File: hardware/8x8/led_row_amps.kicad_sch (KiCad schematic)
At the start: 10 parts

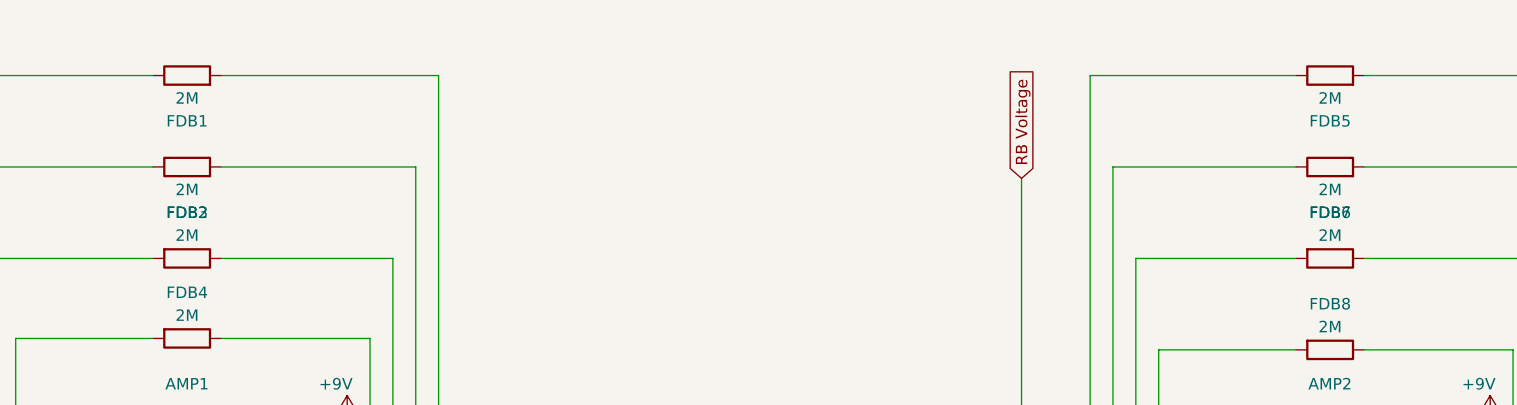
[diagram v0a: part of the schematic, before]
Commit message: Completed Major Routing
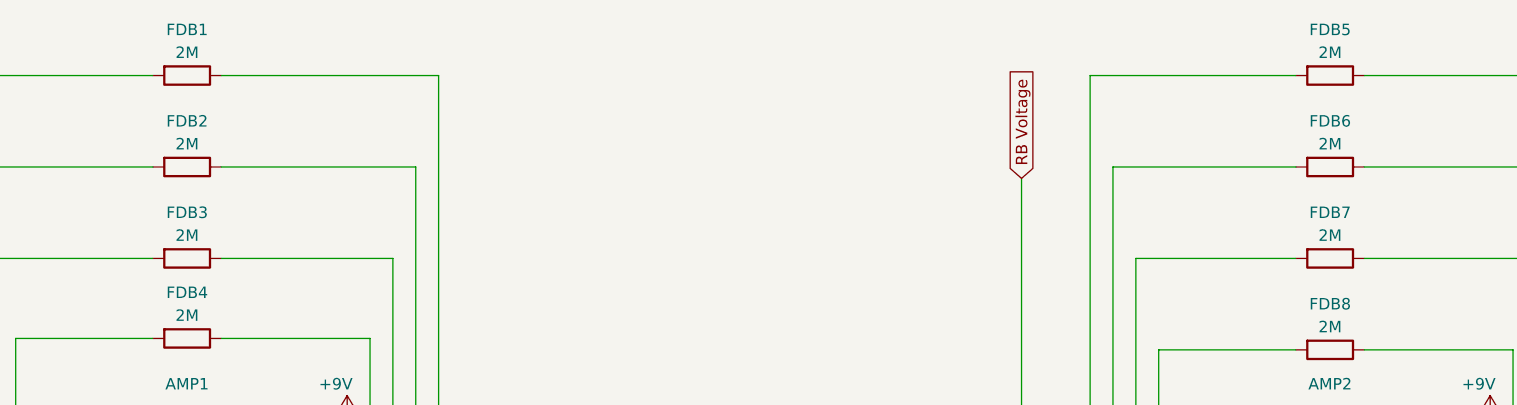
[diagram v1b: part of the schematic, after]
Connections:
- net Amp_IP_1: now also FDB1.2; no longer FDB1.1
- net Amp_IP_2: now also FDB2.2; no longer FDB2.1
- net Amp_IP_5: now also FDB5.2; no longer FDB5.1
- net Amp_IP_6: now also FDB6.2; no longer FDB6.1
- net Amp_OP_1: now also FDB1.1; no longer FDB1.2
- net Amp_OP_2: now also FDB2.1; no longer FDB2.2
- net Amp_OP_5: now also FDB5.1; no longer FDB5.2
- net Amp_OP_6: now also FDB6.1; no longer FDB6.2
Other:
- moved on the sheet: FDB1, FDB2, FDB5, FDB6
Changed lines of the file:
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@@
     (effects (font (size 1.27 1.27)) (justify left))
   )
-  (symbol (lib_id "Device:R") (at 76.2 36.83 90) (unit 1)
+  (symbol (lib_id "Device:R") (at 76.2 36.83 270) (unit 1)
     (in_bom yes) (on_board yes)
-    (property "Reference" "FDB2" (id 0) (at 76.2 41.91 90))
-    (property "Value" "2M" (id 1) (at 76.2 39.37 90))
-    (property "Footprint" "Resistor TH:footprints" (id 2) (at 76.2 38.608 90)
+    (property "Reference" "FDB2" (id 0) (at 76.2 31.75 90))
+    (property "Value" "2M" (id 1) (at 76.2 34.29 90))
+    (property "Footprint" "Resistor TH:footprints" (id 2) (at 76.2 35.052 90)
       (effects (font (size 1.27 1.27)) hide)
     )
@@
     (pin "2")
   )
-  (symbol (lib_id "Device:R") (at 203.2 36.83 90) (unit 1)
+  (symbol (lib_id "Device:R") (at 203.2 36.83 270) (unit 1)
     (in_bom yes) (on_board yes)
-    (property "Reference" "FDB6" (id 0) (at 203.2 41.91 90))
-    (property "Value" "2M" (id 1) (at 203.2 39.37 90))
-    (property "Footprint" "Resistor TH:footprints" (id 2) (at 203.2 38.608 90)
+    (property "Reference" "FDB6" (id 0) (at 203.2 31.75 90))
+    (property "Value" "2M" (id 1) (at 203.2 34.29 90))
+    (property "Footprint" "Resistor TH:footprints" (id 2) (at 203.2 35.052 90)
       (effects (font (size 1.27 1.27)) hide)
     )
@@
   (symbol (lib_id "power:+5V") (at 220.98 95.25 0) (unit 1)
     (in_bom yes) (on_board yes)
-    (property "Reference" "#PWR0103" (id 0) (at 220.98 99.06 0)
+    (property "Reference" "#PWR0101" (id 0) (at 220.98 99.06 0)
       (effects (font (size 1.27 1.27)) hide)
     )
@@
   (symbol (lib_id "power:+9V") (at 93.98 64.77 0) (unit 1)
     (in_bom yes) (on_board yes)
-    (property "Reference" "#PWR0101" (id 0) (at 93.98 68.58 0)
+    (property "Reference" "#PWR0103" (id 0) (at 93.98 68.58 0)
       (effects (font (size 1.27 1.27)) hide)
     )
@@
     (pin "1")
   )
-  (symbol (lib_id "Device:R") (at 203.2 26.67 90) (unit 1)
+  (symbol (lib_id "Device:R") (at 203.2 26.67 270) (unit 1)
     (in_bom yes) (on_board yes)
-    (property "Reference" "FDB5" (id 0) (at 203.2 31.75 90))
-    (property "Value" "2M" (id 1) (at 203.2 29.21 90))
-    (property "Footprint" "Resistor TH:footprints" (id 2) (at 203.2 28.448 90)
+    (property "Reference" "FDB5" (id 0) (at 203.2 21.59 90))
+    (property "Value" "2M" (id 1) (at 203.2 24.13 90))
+    (property "Footprint" "Resistor TH:footprints" (id 2) (at 203.2 24.892 90)
       (effects (font (size 1.27 1.27)) hide)
     )
@@
     (pin "2")
   )
-  (symbol (lib_id "Device:R") (at 76.2 26.67 90) (unit 1)
+  (symbol (lib_id "Device:R") (at 76.2 26.67 270) (unit 1)
     (in_bom yes) (on_board yes)
-    (property "Reference" "FDB1" (id 0) (at 76.2 31.75 90))
-    (property "Value" "2M" (id 1) (at 76.2 29.21 90))
-    (property "Footprint" "Resistor TH:footprints" (id 2) (at 76.2 28.448 90)
+    (property "Reference" "FDB1" (id 0) (at 76.2 21.59 90))
+    (property "Value" "2M" (id 1) (at 76.2 24.13 90))
+    (property "Footprint" "Resistor TH:footprints" (id 2) (at 76.2 24.892 90)
       (effects (font (size 1.27 1.27)) hide)
     )
@@
   (symbol (lib_id "power:+5V") (at 93.98 95.25 0) (unit 1)
     (in_bom yes) (on_board yes)
-    (property "Reference" "#PWR0102" (id 0) (at 93.98 99.06 0)
+    (property "Reference" "#PWR0104" (id 0) (at 93.98 99.06 0)
       (effects (font (size 1.27 1.27)) hide)
     )
@@
   (symbol (lib_id "power:+9V") (at 220.98 64.77 0) (unit 1)
     (in_bom yes) (on_board yes)
-    (property "Reference" "#PWR0104" (id 0) (at 220.98 68.58 0)
+    (property "Reference" "#PWR0102" (id 0) (at 220.98 68.58 0)
       (effects (font (size 1.27 1.27)) hide)
     )
